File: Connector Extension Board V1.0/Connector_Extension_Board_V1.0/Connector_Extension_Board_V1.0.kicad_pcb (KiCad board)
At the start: 4 copper layers, 67.7 x 69 mm, 65 parts, among them J1 1723103104, U10 TPS259571DSGR, U11 TPS259571DSGR, U12 TPS259571DSGR, U3 TPS259571DSGR, U4 TPS259571DSGR, U5 TPS259571DSGR, U8 TPS259571DSGR, U9 TPS1HC30BQPWPRQ1

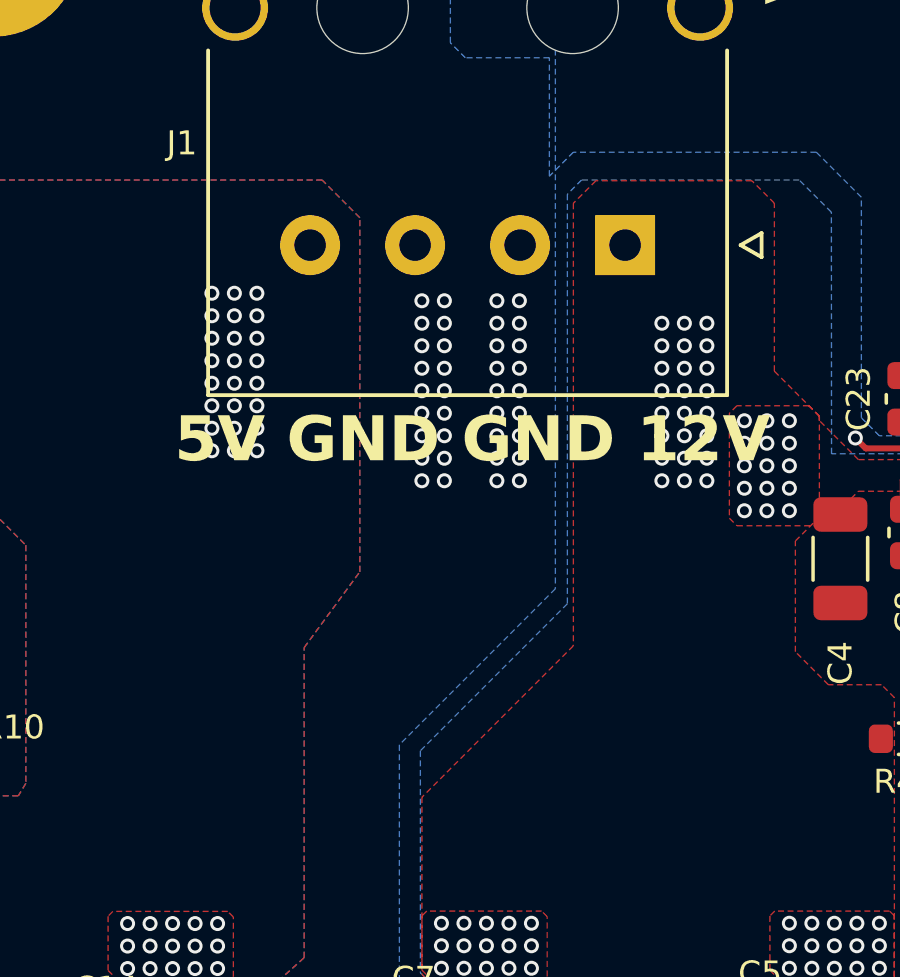
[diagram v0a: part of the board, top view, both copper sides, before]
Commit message: cap nhat 26/2
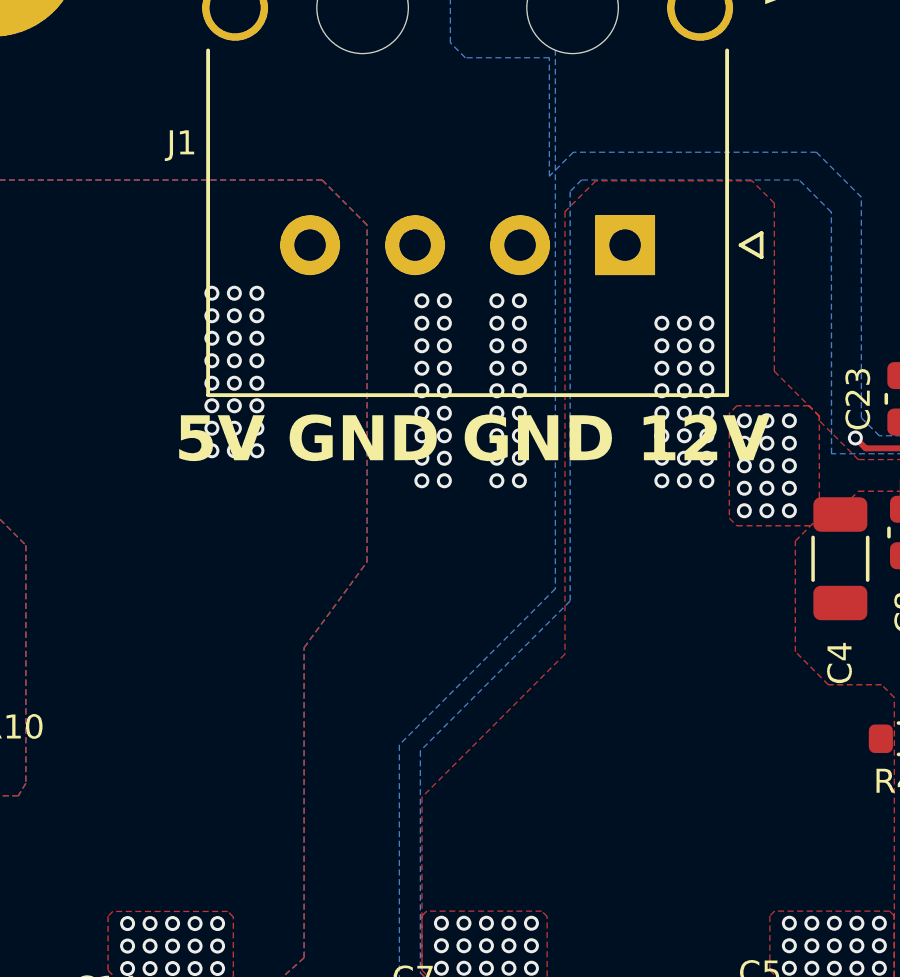
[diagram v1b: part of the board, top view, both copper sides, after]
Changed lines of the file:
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@@
 			(disableapertmacros no)
 			(usegerberextensions yes)
-			(usegerberattributes yes)
+			(usegerberattributes no)
 			(usegerberadvancedattributes no)
 			(creategerberjobfile no)
@@
 			(psa4output no)
 			(plot_black_and_white yes)
-			(plotinvisibletext no)
 			(sketchpadsonfab no)
 			(plotpadnumbers no)
@@
 			(pinfunction "Pin_2")
 			(pintype "passive")
+			(zone_connect 1)
+			(thermal_bridge_width 0.8)
+			(thermal_gap 0.3)
 		)
 		(pad "3" thru_hole circle
@@
 			(pinfunction "Pin_3")
 			(pintype "passive")
+			(zone_connect 1)
+			(thermal_bridge_width 0.8)
+			(thermal_gap 0.3)
 		)
 		(pad "4" thru_hole circle
@@
 		(hatch edge 0.5)
 		(connect_pads
-			(clearance 0.4)
+			(clearance 0.5)
 		)
 		(min_thickness 0.2)
@@
 		(layer "F.Cu")
 		(hatch edge 0.5)
+		(priority 1)
 		(connect_pads
 			(clearance 0.3)
@@
 		(polygon
 			(pts
-				(xy 132.352 75.6998) (xy 127.3045 80.7473) (xy 127.3045 86.5148) (xy 127.7895 86.9998) (xy 131.4345 86.9998)
+				(xy 132.072 75.9798) (xy 127.3045 80.7473) (xy 127.3045 86.5148) (xy 127.7895 86.9998) (xy 131.4345 86.9998)
 				(xy 131.4795 87.0448) (xy 143.052 87.0448) (xy 143.052 77.4273) (xy 142.6245 76.9998) (xy 140.852 76.9998)
 				(xy 139.752 75.8998) (xy 139.752 72.2098) (xy 140.552 71.4098) (xy 140.552 68.0498) (xy 139.052 66.5498)
-				(xy 139.052 60.9498) (xy 138.302 60.1998) (xy 133.102 60.1998) (xy 132.352 60.9498)
+				(xy 139.052 60.9498) (xy 138.302 60.1998) (xy 133.102 60.1998) (xy 132.072 61.2298)
 			)
 		)
@@
 				(xy 114.102 72.3498) (xy 114.102 80.283133) (xy 113.852 80.6998) (xy 109.702 80.6998) (xy 105.602 84.7998)
 				(xy 105.602 86.5498) (xy 106.452 87.3998) (xy 122.034402 87.308139) (xy 123.377 86.099801) (xy 123.377 75.763631)
-				(xy 125.234783 73.233883) (xy 125.234783 61.432583) (xy 123.978596 60.176396)
+				(xy 125.474783 72.907075) (xy 125.474783 61.672583) (xy 123.978596 60.176396)
 			)
 		)
@@
 		(polygon
 			(pts
-				(xy 132.152 60.6498) (xy 132.152 74.2998) (xy 127.252 79.1998) (xy 127.252 86.5998) (xy 129.452 88.7998)
+				(xy 132.242 60.5598) (xy 132.242 74.2098) (xy 127.252 79.1998) (xy 127.252 86.5998) (xy 129.452 88.7998)
 				(xy 144.452 88.7998) (xy 154.652 88.7998) (xy 156.852 90.9998) (xy 156.852 94.4998) (xy 153.752 97.5998)
 				(xy 153.752 101.2998) (xy 153.952 101.4998) (xy 165.150171 101.4998) (xy 165.848043 100.801928)
